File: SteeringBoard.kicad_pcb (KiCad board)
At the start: 2 copper layers, 41.8 x 28 mm, 55 parts, among them J1 SWD, J2 Conn_01x02_Pin, J3 Conn_02x05_Counter_Clockwise, J4 Conn_01x04_Pin, SW1 Reset, U1 STM32L431CBTx, U2 ISO1044BD, U3 CDSOT23-T24CAN, U4 TPS562231DRLR, U5 RO-123.3S

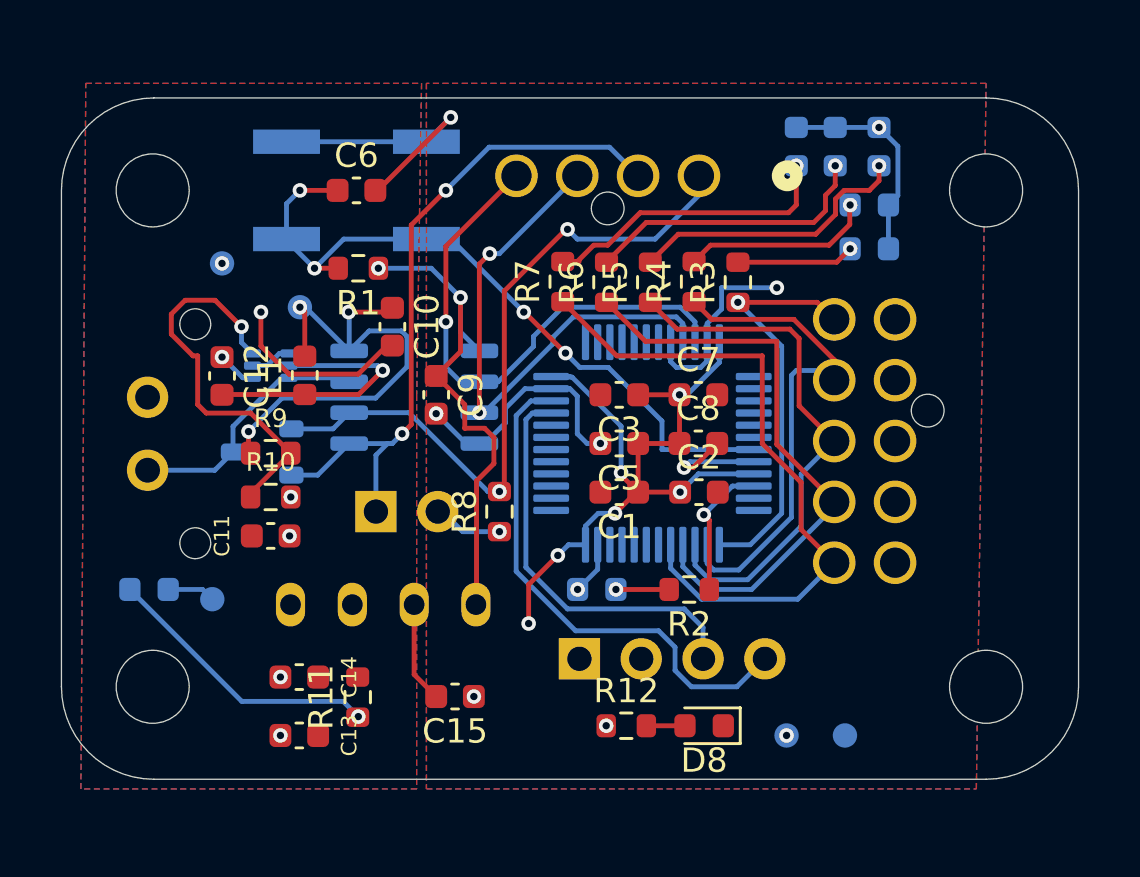
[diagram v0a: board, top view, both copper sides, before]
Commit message: final
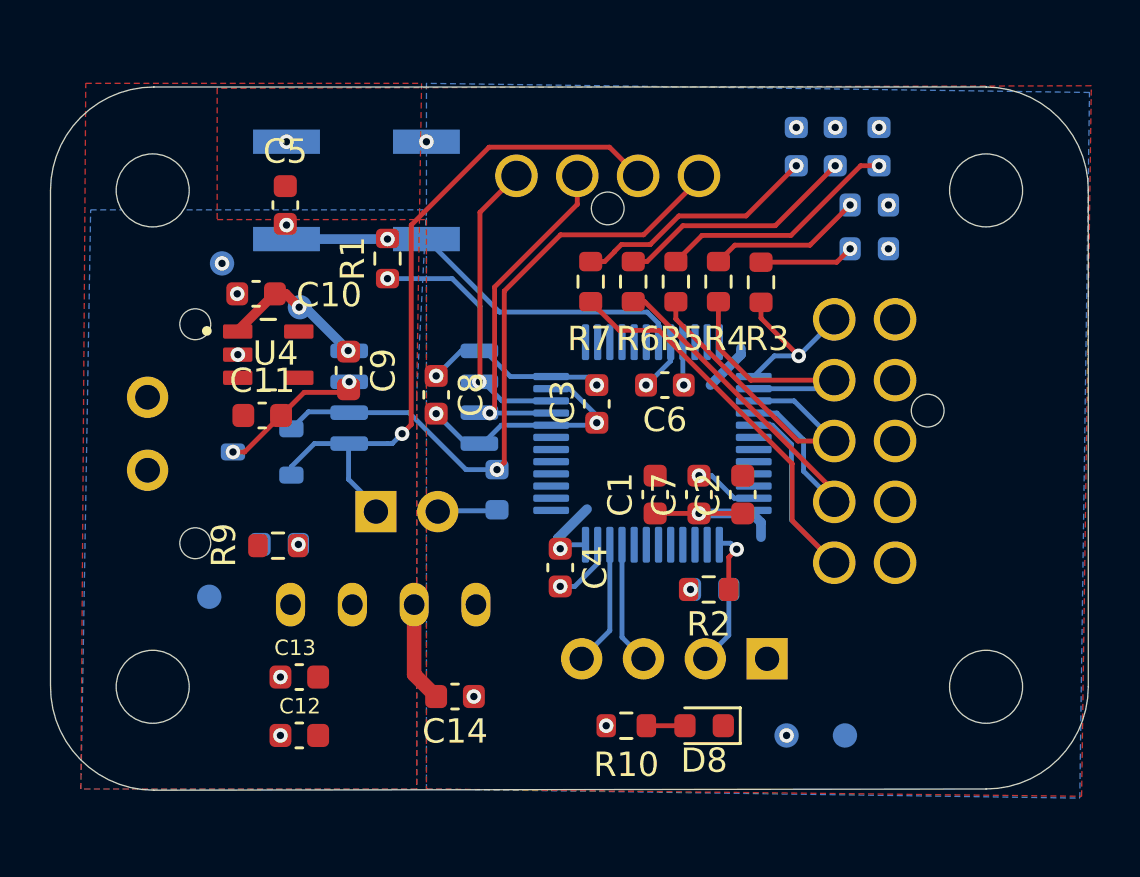
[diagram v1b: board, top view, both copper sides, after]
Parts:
- removed the C12 at (128.6, 92.6)
- removed L1: 3.3uH, Inductor_SMD:L_0603_1608Metric
- removed the R10 at (130.6, 97.6)
- removed the R9 at (130.6, 95.8)
- added C10: 1nF, Capacitor_SMD:C_0603_1608Metric, F.Cu at (130.0, 89.2)
- C11: value 10uF -> 100nF
- R8: moved to B.Cu
- U4: value TPS562231DRLR -> TLV70130DBVR; footprint Package_TO_SOT_SMD:SOT-563 -> UTSVT_Power:SOT95P280X145-5N; moved to F.Cu
- moved J1 7.71 mm to (151.0, 104.2), turned to 90 degrees
- moved R9 7.03 mm to (130.9, 99.6), turned to 0 degrees
- moved D7 5.66 mm to (130.9, 99.5), turned to 0 degrees
- moved C4 5.65 mm to (142.5, 100.5), turned to -90 degrees
- moved C11 4.96 mm to (130.2, 94.2)
- moved D1 4.64 mm to (148.6, 101.4), turned to 180 degrees
- moved C5 2.99 mm to (131.2, 85.6), turned to 90 degrees
- moved C9 2.55 mm to (133.8, 92.4)
- moved C7 2.10 mm to (148.2, 97.5), turned to 90 degrees
- moved C2 1.80 mm to (150.0, 97.5), turned to 90 degrees
- moved C1 1.48 mm to (146.4, 97.5), turned to 90 degrees
- moved C6 1.43 mm to (146.8, 93.0), turned to 180 degrees
- moved R1 1.26 mm to (135.4, 87.8), turned to 90 degrees
- moved R7 1.15 mm to (143.8, 88.8)
- moved R6 1.10 mm to (145.5, 88.8)
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- renumbered C13 to C12, C14 to C13, C15 to C14, C5 to C4, C6 to C5, C7 to C6, C8 to C7, C9 to C8, C10 to C9, R12 to R10, R11 to R9
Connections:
- C11 pad 1: /12V_Ext -> +12V
- U1 pad 10: /PA0 -> unconnected-(U1-PA0-Pad10)
- U1 pad 25: unconnected-(U1-PB12-Pad25) -> /PA0
- U4 pad 1: /12V_Ext -> /3V3_Bus
- U4 pad 2: /PowerDist/SW -> GNDPWR
- U4 pad 3: GNDPWR -> +12V
- U4 pad 4: /PowerDist/BST -> unconnected-(U4-NC-Pad4)
- U4 pad 5: /12V_Ext -> unconnected-(U4-NC-Pad5)
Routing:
- net GND: track 49.0 -> 24.5 mm, vias 8 -> 13
- net +3.3V: track 51.4 -> 27.6 mm, vias 10 -> 8
- net /SWCLK: track 21.3 -> 5.17 mm
- net /PowerDist/FB: track 16.1 -> 0.00 mm, vias 1 -> 0
- net /3V3_Bus: track 20.3 -> 6.21 mm, vias 3 -> 2
- net GNDPWR: track 19.8 -> 6.29 mm, vias 5 -> 6
- net /SWDIO: track 16.8 -> 5.05 mm
- net Net-(D7-A): track 11.6 -> 0.00 mm
- net /PowerDist/SW: track 10.9 -> 0.00 mm, vias 1 -> 0
- net /CAN_TX: track 22.1 -> 12.2 mm
- net /NRST: track 28.2 -> 18.3 mm, vias 4 -> 2
- net /RGEN_E-: track 16.8 -> 7.15 mm
- net /CRS_SET-: track 20.1 -> 10.7 mm
- net /CAN_RX: track 22.5 -> 13.8 mm, vias 2 -> 1
- net /REG-: track 22.0 -> 13.3 mm
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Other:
- board size 41.8 x 28 mm -> 42.6 x 28.9 mm

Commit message: fixed the switch
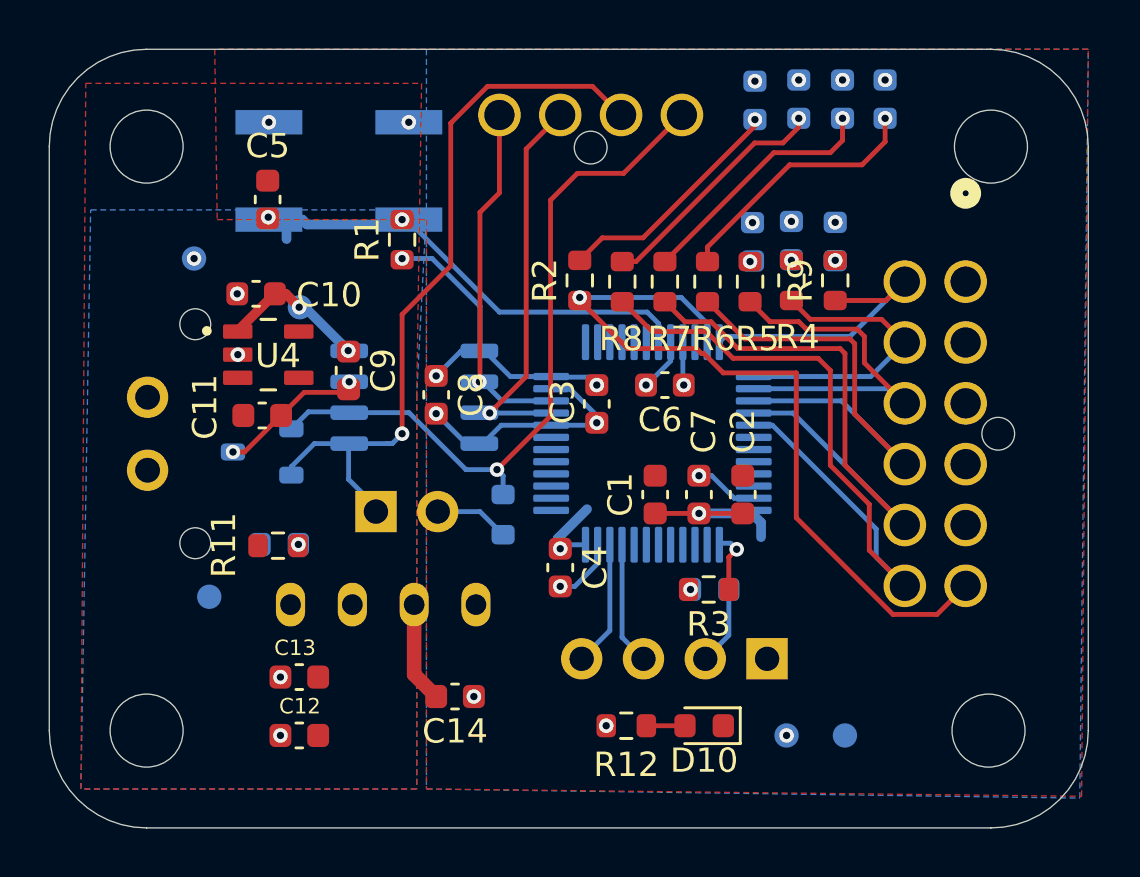
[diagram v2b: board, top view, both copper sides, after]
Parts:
- removed the J3 at (156.3, 90.3)
- added D1: LED, LED_SMD:LED_0603_1608Metric, B.Cu at (150.5, 81.3)
- added D8: LED, LED_SMD:LED_0603_1608Metric, B.Cu at (153.8, 87.1)
- added J2: Conn_02x06_Counter_Clockwise, UTSVT_Connectors:CONN_SD-105310-100_12_MOL, B.Cu at (159.2, 88.8)
- added R2: R_US, Resistor_SMD:R_0603_1608Metric, F.Cu at (143.3, 88.7)
- added R9: R_US, Resistor_SMD:R_0603_1608Metric, F.Cu at (153.8, 88.7)
- moved D4 5.03 mm to (150.4, 87.1), turned to -90 degrees
- moved D3 3.22 mm to (152.0, 87.1), turned to -90 degrees
- moved J5 2.60 mm to (147.5, 81.9)
- moved D6 1.97 mm to (154.1, 81.2)
- moved D5 1.97 mm to (155.8, 81.2)
- moved D7 1.95 mm to (152.3, 81.2)
- moved MH2 1.82 mm to (125.5, 83.2)
- moved MH3 1.82 mm to (125.5, 107.2)
- moved MH1 1.81 mm to (160.2, 83.2)
- moved MH4 1.80 mm to (160.1, 107.2)
- moved R5 1.30 mm to (150.3, 88.8)
- moved R6 1.30 mm to (148.6, 88.8)
- moved R7 1.30 mm to (146.8, 88.8)
- moved R8 1.30 mm to (145.1, 88.8)
- moved R4 1.25 mm to (152.0, 88.7)
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- renumbered D8 to D10, D1 to D2, D2 to D3, D3 to D4, D4 to D5, D5 to D6, D6 to D7, D7 to D9, J2 to J3, J4 to J5, R8 to R10, R9 to R11, R10 to R12, R2 to R3, R3 to R4, R4 to R5, R5 to R6, R6 to R7, R7 to R8
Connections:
- net /REG- renamed /CEN-
- net /TSS- renamed /TSSL-
- U1 pad 11: unconnected-(U1-PA1-Pad11) -> /TSSR-
- U1 pad 12: unconnected-(U1-PA2-Pad12) -> /TSSO-
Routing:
- net /TSSR-: track 0.00 -> 31.6 mm, vias 0 -> 1
- net /TSSO-: track 0.00 -> 11.8 mm
- net Net-(D1-A): track 0.00 -> 9.75 mm, vias 0 -> 1
- net /TSSL-: track 17.5 -> 24.5 mm
- net /CEN-: track 13.3 -> 19.9 mm
- net Net-(D4-A): track 6.38 -> 0.00 mm
- net /HRN_PD-: track 23.3 -> 29.5 mm
- net /RGEN_E-: track 7.15 -> 12.2 mm, vias 1 -> 0
- net /CRS_SET-: track 10.7 -> 15.2 mm
- net Net-(D3-A): track 3.89 -> 0.00 mm
- net /CAN_H: track 27.2 -> 29.7 mm
- net +3.3V: track 27.6 -> 25.4 mm
- net /CAN_RX: track 13.8 -> 16.0 mm
- net /CAN_TX: track 12.2 -> 14.4 mm
- net /CAN_L: track 28.4 -> 30.2 mm
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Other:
- board size 42.6 x 28.9 mm -> 42.7 x 32 mm
